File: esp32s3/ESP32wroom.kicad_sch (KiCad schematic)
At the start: 64 parts, among them J1 USB_C_Receptacle_USB2.0, J2 CAMERA, J3 Conn_01x02, J4 Conn-01x02_P2mm_NONAME_JST-PH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, J5 Conn_01x19, J6 Conn_01x20, SW1 SW_SPST, SW2 SW_SPST, U1 AMS1117-3.3, U2 ESP32-S3-WROOM-1, U3 ME6206A15XG, U4 ME6206A28XG, U5 CH9102F, U6 PCF85063AT, U7 TP4057-42-SOT26-R, Y1 32.768kHz_Q13FC1350000400

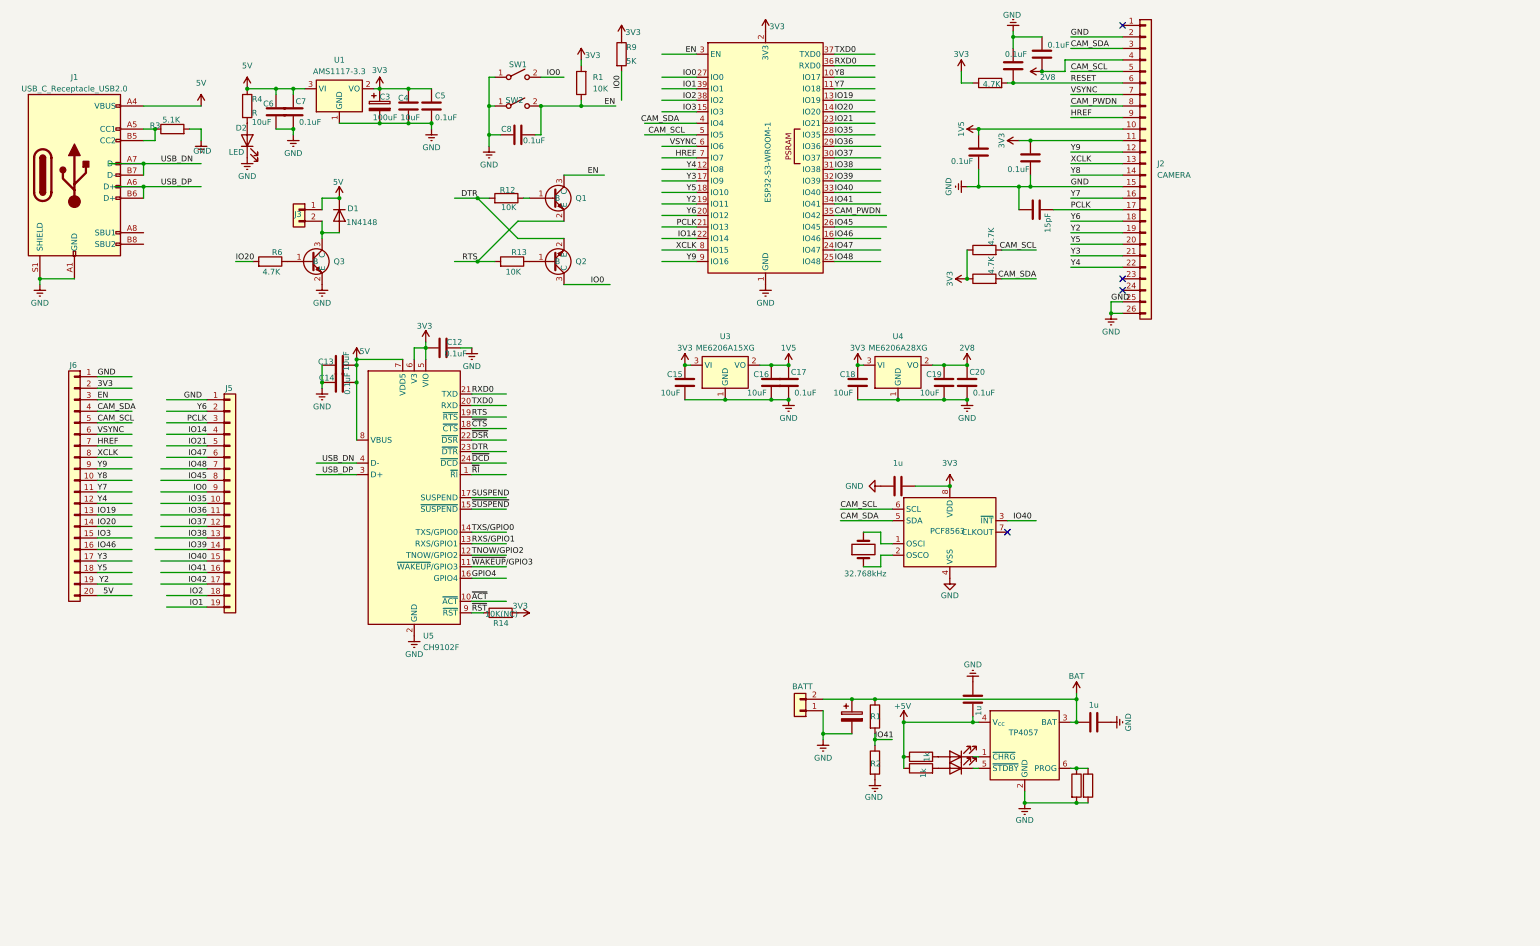
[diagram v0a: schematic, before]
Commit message: 添加图片
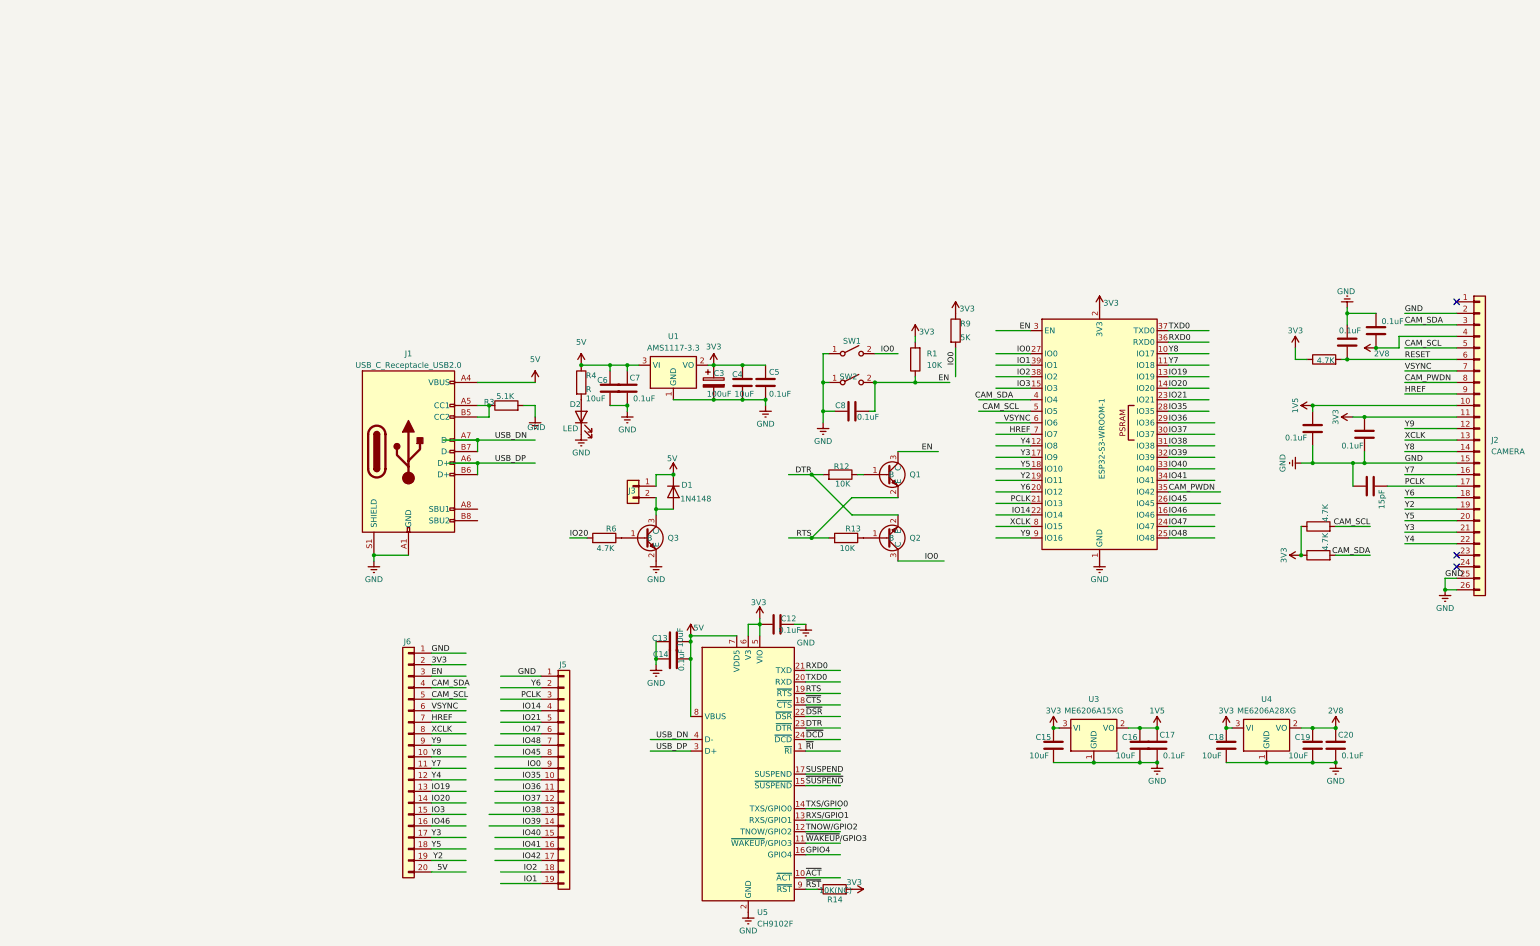
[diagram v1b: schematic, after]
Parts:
- removed C21, C23, C24: 10u_0402_CL05A105KA5NQNC, Capacitor_SMD:C_0402_1005Metric, symbol 00-kiml-capacitors-smd:1u_0402_CL05A105KA5NQNC
- removed C22: 100u_CASE-B-3528_TAJB107K006RNJ, 00-kiml-capacitor-tantalum:CP_EIA-3528-15_AVX-H, symbol 00-kiml-capacitors-smd:100u_CASE-B-3528_TAJB107K006RNJ
- removed D3, D4: LED, LED_SMD:LED_0603_1608Metric, symbol Device:LED
- removed J4: Conn-01x02_P2mm_NONAME_JST-PH_C47647, 00-kiml-connector-jst:JST_PH_S2B-PH-SM4-TB_1x02-1MP_P2.00mm_Horizontal, symbol 00-kiml-connector-jst:Conn-01x02_P2.0mm_NONAME_JST-PH_C47647
- removed R1, R2: 976k_0402_0402WGD9763TCE, Resistor_SMD:R_0402_1005Metric, symbol 00-kiml-resistors-smd:976k_0402_0402WGD9763TCE
- removed R17, R18, R19, R20: 10k_0402_0402WGF1002TCE, Resistor_SMD:R_0402_1005Metric, symbol 00-kiml-resistors-smd:10k_0402_0402WGF1002TCE
- removed U6: PCF85063AT, Package_SO:SO-8_3.9x4.9mm_P1.27mm, symbol 00-kiml-timer-rtc:PCF85063AT/AAZ
- removed U7: TP4057-42-SOT26-R, Package_TO_SOT_SMD:SOT-23-6, symbol 00-kiml-battery-management:TP4057-42-SOT26-R
- removed Y1: 32.768kHz_Q13FC1350000400, 00-kiml-crystal-smd:Crystal_SMD_3215-2Pin_3.2x1.5mm, symbol 00-kiml-crystal:32.768kHz_Q13FC1350000400
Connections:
- no-connect marks 4 -> 3
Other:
- moved on the sheet: C12, C13, C14, C15, C16, C17, C18, C19, C20, C3, C4, C5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
